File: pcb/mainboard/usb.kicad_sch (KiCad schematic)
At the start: 9 parts, among them J801 USB_B_Mini, U201 MIMX8MN6DVTJZAA, U802 USBLC6-2P6

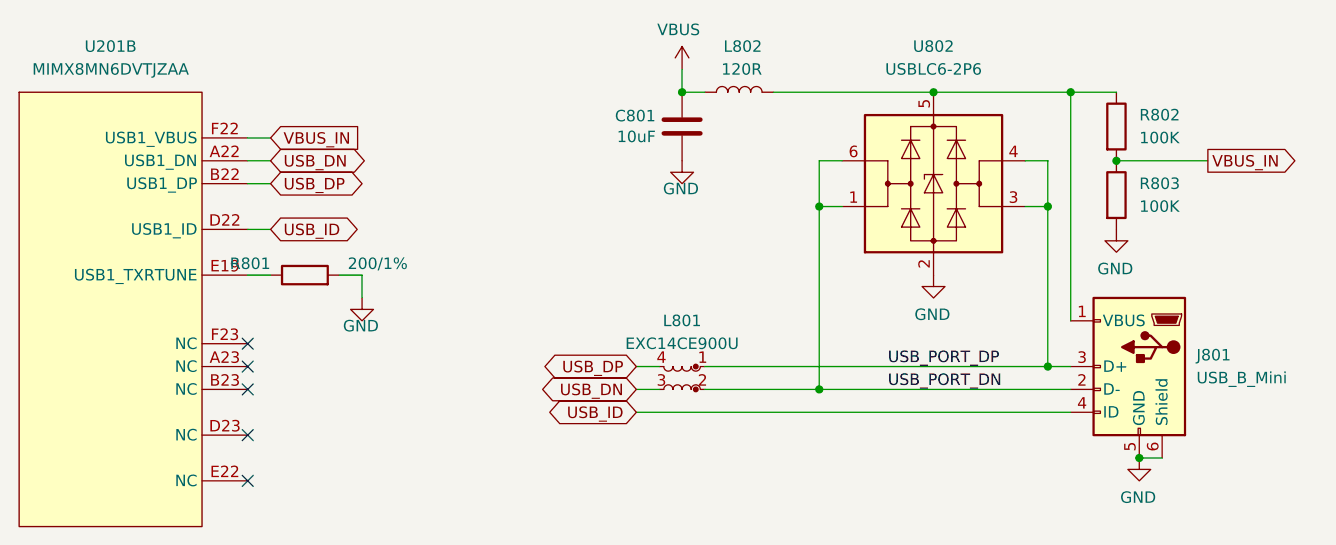
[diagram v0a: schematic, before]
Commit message: Keypad bugfix, pulling in submodules
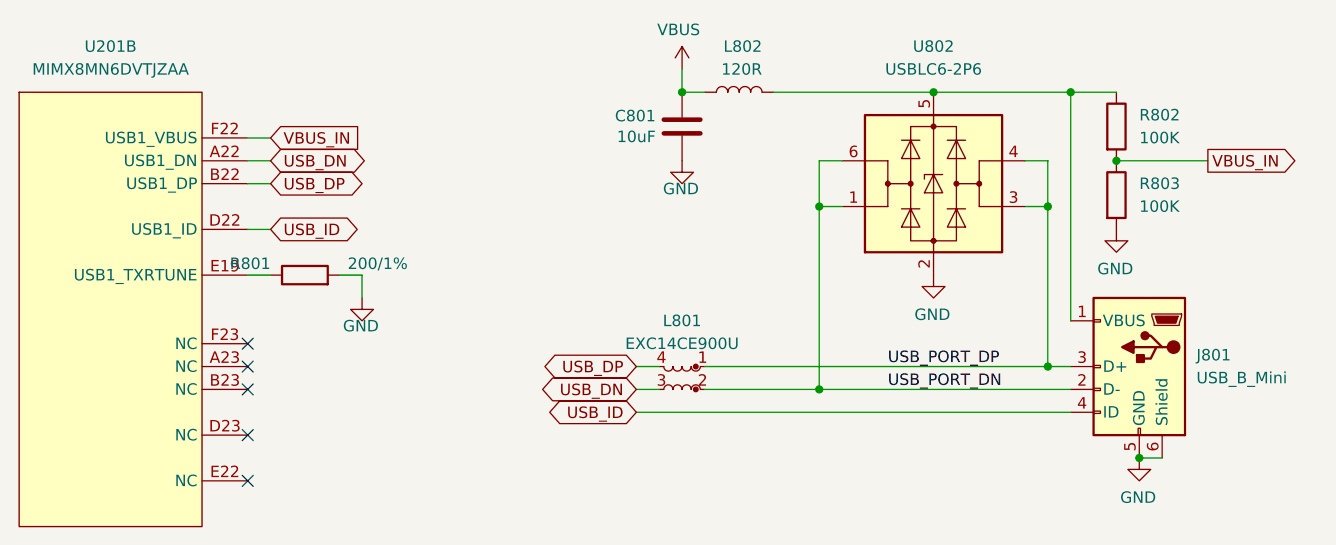
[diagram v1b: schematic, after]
